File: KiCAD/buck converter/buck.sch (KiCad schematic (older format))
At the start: 16 parts, among them P1 VIN, P2 VOUT, Q1 Q_PMOS_DGS, U1 LTC1771

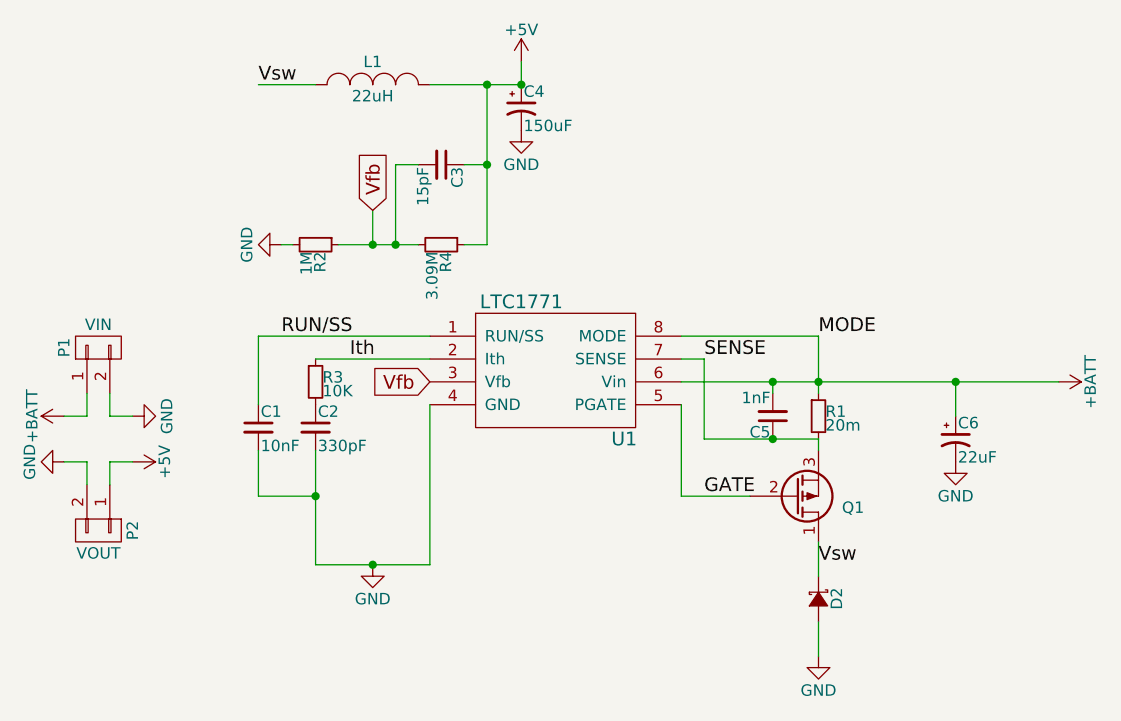
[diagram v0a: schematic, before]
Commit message: Updated board layout
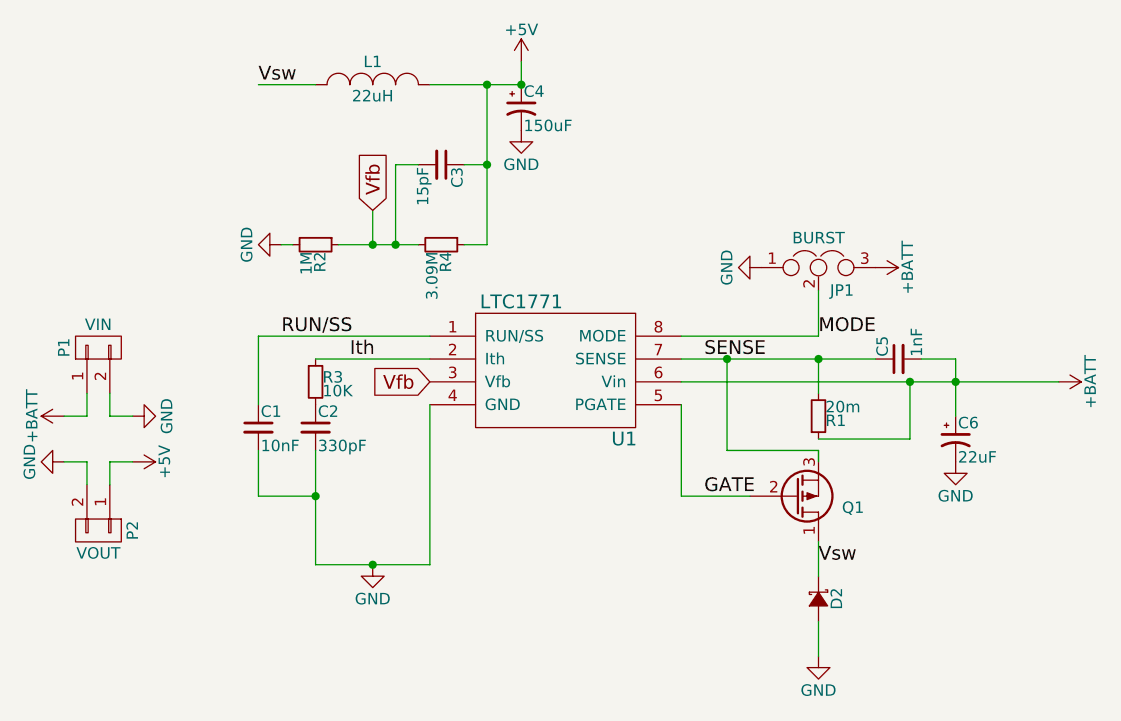
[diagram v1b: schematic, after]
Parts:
- added JP1: BURST, Connectors:PINHEAD1-3, symbol Jumper_NC_Dual
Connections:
- net +BATT: now also JP1.3; no longer U1.8 (MODE)
- net GND: now also JP1.1
- new net MODE: JP1.2, U1.8 (MODE)
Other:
- moved on the sheet: C5
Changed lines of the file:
@@
 F 3 "" H 6900 4050 50  0000 C CNN
 	1    6900 4050
-	1    0    0    -1
+	1    0    0    1
 $EndComp
 $Comp
@@
 L C_Small C5
 U 1 1 58964849
-P 6700 4050
-F 0 "C5" H 6710 4120 50  0000 L CNN
-F 1 "1nF" H 6710 3970 50  0000 L CNN
-F 2 "Capacitors_SMD:C_0805_HandSoldering" H 6700 4050 50  0001 C CNN
-F 3 "" H 6700 4050 50  0000 C CNN
-	1    6700 4050
-	-1   0    0    1
+P 7250 3800
+F 0 "C5" H 7260 3870 50  0000 L CNN
+F 1 "1nF" H 7260 3720 50  0000 L CNN
+F 2 "Capacitors_SMD:C_0805_HandSoldering" H 7250 3800 50  0001 C CNN
+F 3 "" H 7250 3800 50  0000 C CNN
+	1    7250 3800
+	0    -1   -1   0
 $EndComp
 $Comp
@@
 Connection ~ 7500 3900
 Wire Wire Line
-	7500 3900 7500 4050
+	7500 3800 7500 4050
 Wire Wire Line
 	6300 4000 6300 4400
@@
 	6300 4400 6600 4400
 Wire Wire Line
-	6900 3700 6900 3950
-Connection ~ 6900 3900
-Wire Wire Line
-	6900 4150 6900 4200
-Wire Wire Line
-	6400 4150 6400 3800
-Wire Wire Line
-	6400 3800 6300 3800
+	6300 3800 7150 3800
 Wire Wire Line
 	6900 4750 6900 4600
 $Comp
-L GND #PWR06
+L GND #PWR05
 U 1 1 589662F9
 P 7500 4250
-F 0 "#PWR06" H 7500 4000 50  0001 C CNN
+F 0 "#PWR05" H 7500 4000 50  0001 C CNN
 F 1 "GND" H 7500 4100 50  0000 C CNN
 F 2 "" H 7500 4250 50  0000 C CNN
@@
 Wire Wire Line
 	6300 3700 6900 3700
-Connection ~ 6700 3900
-Wire Wire Line
-	6700 3950 6700 3900
-Wire Wire Line
-	6400 4150 6900 4150
-Connection ~ 6700 4150
 Wire Wire Line
 	4700 3800 5200 3800
@@
 Connection ~ 4950 3300
 $Comp
-L GND #PWR08
+L GND #PWR06
 U 1 1 58967FFD
 P 4550 3300
-F 0 "#PWR08" H 4550 3050 50  0001 C CNN
+F 0 "#PWR06" H 4550 3050 50  0001 C CNN
 F 1 "GND" H 4550 3150 50  0000 C CNN
 F 2 "" H 4550 3300 50  0000 C CNN
@@
 Connection ~ 5450 2600
 $Comp
-L GND #PWR09
+L GND #PWR07
 U 1 1 58968BDB
 P 5600 2800
-F 0 "#PWR09" H 5600 2550 50  0001 C CNN
+F 0 "#PWR07" H 5600 2550 50  0001 C CNN
 F 1 "GND" H 5600 2650 50  0000 C CNN
 F 2 "" H 5600 2800 50  0000 C CNN
@@
 	5200 2600 5600 2600
 $Comp
-L +5V #PWR010
+L +5V #PWR08
 U 1 1 58969042
 P 5600 2500
-F 0 "#PWR010" H 5600 2350 50  0001 C CNN
+F 0 "#PWR08" H 5600 2350 50  0001 C CNN
 F 1 "+5V" H 5600 2640 50  0000 C CNN
 F 2 "" H 5600 2500 50  0000 C CNN
@@
 	5600 2600 5600 2500
 $Comp
-L +5V #PWR011
+L +5V #PWR09
 U 1 1 589690C9
 P 3900 4250
-F 0 "#PWR011" H 3900 4100 50  0001 C CNN
+F 0 "#PWR09" H 3900 4100 50  0001 C CNN
 F 1 "+5V" H 3900 4390 50  0000 C CNN
 F 2 "" H 3900 4250 50  0000 C CNN
@@
 	3800 4250 3900 4250
 $Comp
-L GND #PWR012
+L GND #PWR010
 U 1 1 5896914A
 P 3600 4250
-F 0 "#PWR012" H 3600 4000 50  0001 C CNN
+F 0 "#PWR010" H 3600 4000 50  0001 C CNN
 F 1 "GND" H 3600 4100 50  0000 C CNN
 F 2 "" H 3600 4250 50  0000 C CNN
@@
 	6900 5100 6900 4950
 $Comp
-L GND #PWR05
+L GND #PWR011
 U 1 1 58965DDE
 P 6900 5100
-F 0 "#PWR05" H 6900 4850 50  0001 C CNN
+F 0 "#PWR011" H 6900 4850 50  0001 C CNN
 F 1 "GND" H 6900 4950 50  0000 C CNN
 F 2 "" H 6900 5100 50  0000 C CNN
@@
 Text Label 4550 3700 0    60   ~ 0
 RUN/SS
+$Comp
+L Jumper_NC_Dual JP1
+U 1 1 5898D624
+P 6900 3400
+F 0 "JP1" H 6950 3300 50  0000 L CNN
+F 1 "BURST" H 6900 3500 50  0000 C BNN
+F 2 "Connectors:PINHEAD1-3" H 6900 3400 50  0001 C CNN
+F 3 "" H 6900 3400 50  0000 C CNN
+	1    6900 3400
+	1    0    0    -1
+$EndComp
+$Comp
+L +BATT #PWR012
+U 1 1 5898D713
+P 7150 3400
+F 0 "#PWR012" H 7150 3250 50  0001 C CNN
+F 1 "+BATT" H 7150 3540 50  0000 C CNN
+F 2 "" H 7150 3400 50  0000 C CNN
+F 3 "" H 7150 3400 50  0000 C CNN
+	1    7150 3400
+	0    1    1    0
+$EndComp
+$Comp
+L GND #PWR013
+U 1 1 5898D751
+P 6650 3400
+F 0 "#PWR013" H 6650 3150 50  0001 C CNN
+F 1 "GND" H 6650 3250 50  0000 C CNN
+F 2 "" H 6650 3400 50  0000 C CNN
+F 3 "" H 6650 3400 50  0000 C CNN
+	1    6650 3400
+	0    1    1    0
+$EndComp
+Wire Wire Line
+	6900 3700 6900 3500
+Wire Wire Line
+	6900 3800 6900 3950
+Connection ~ 6900 3800
+Wire Wire Line
+	7350 3800 7500 3800
+Wire Wire Line
+	6900 4250 6900 4200
+Wire Wire Line
+	6900 4200 6500 4200
+Wire Wire Line
+	6500 4200 6500 3800
+Connection ~ 6500 3800
+Wire Wire Line
+	6900 4150 7300 4150
+Wire Wire Line
+	7300 4150 7300 3900
+Connection ~ 7300 3900
 $EndSCHEMATC
